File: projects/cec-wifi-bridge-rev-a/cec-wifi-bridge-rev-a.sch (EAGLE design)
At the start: 56 parts, among them J1 DX4R005HJ5R2000, J3 DEBUG, J4 10029449-001RLF, J5 PROGRAM, T1 MMBT3904, T2 MMBT3904, U1 MCP73831/2/OT, U2 TPS61200DRC, U3 ESP8266EX, U4 SPI-FLASH-SOIC8, X1 26MHz

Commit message: Add part number for ESP8266.
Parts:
- U3: PN (none) -> ESP8266EX
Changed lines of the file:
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@@
 <attribute name="BOM" value="EXCLUDE"/>
 </part>
-<part name="U3" library="espressif" deviceset="ESP8266EX" device=""/>
+<part name="U3" library="espressif" deviceset="ESP8266EX" device="">
+<attribute name="PN" value="ESP8266EX"/>
+</part>
 <part name="X1" library="crystals" deviceset="GROUNDED-CRYSTAL" device="-EPSON-TSX-3225" value="26MHz">
 <attribute name="PN" value="TSX-3225 26.0000MF09Z-AC3"/>
@@
 <attribute name="BOM" x="0" y="0" size="5.08" layer="96" display="off"/>
 </instance>
-<instance part="U3" gate="G$1" x="86.36" y="99.06"/>
+<instance part="U3" gate="G$1" x="86.36" y="99.06">
+<attribute name="PN" x="86.36" y="99.06" size="1.778" layer="96" display="off"/>
+</instance>
 <instance part="X1" gate="G$1" x="198.12" y="121.92">
 <attribute name="PN" x="198.12" y="121.92" size="1.778" layer="96" display="off"/>

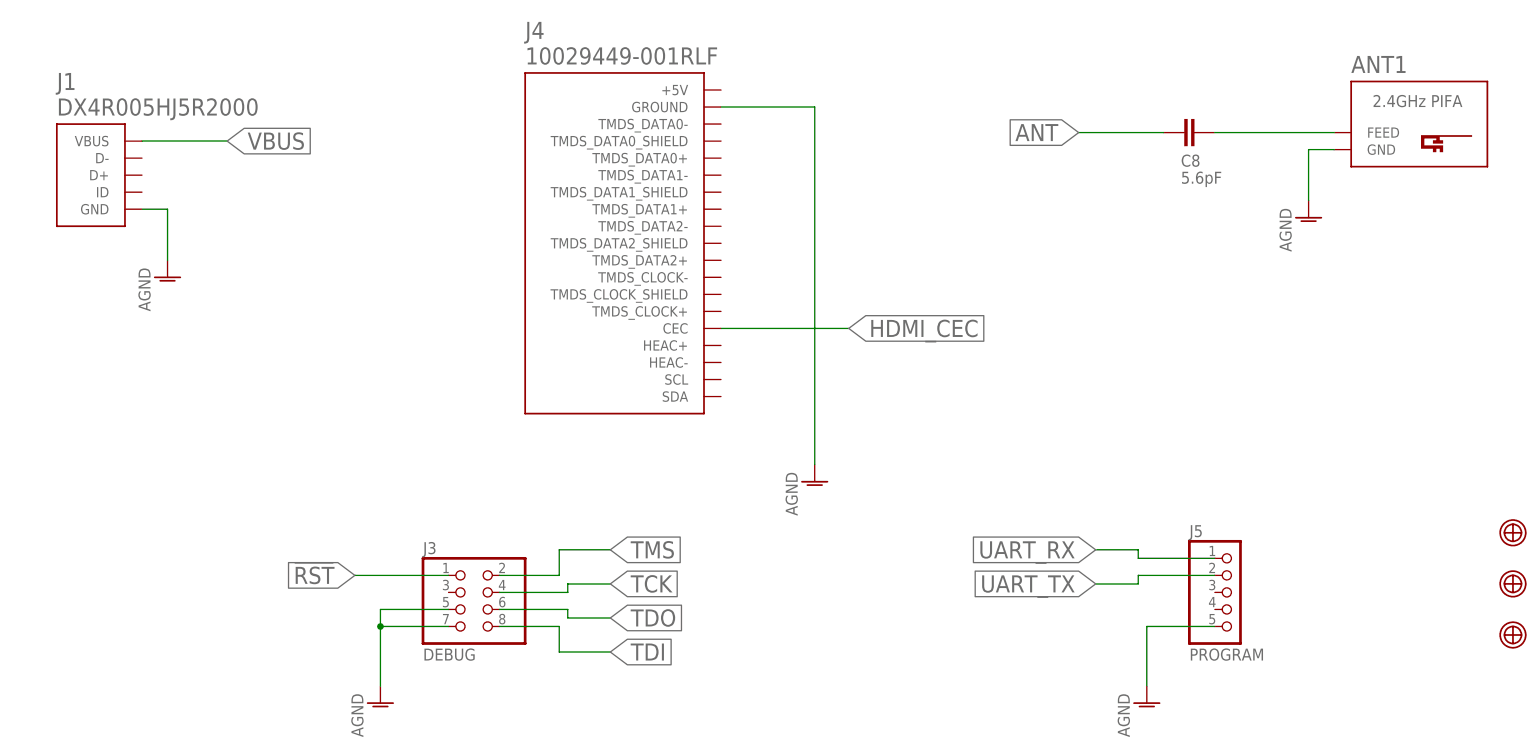
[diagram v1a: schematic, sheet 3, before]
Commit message: Add testpoints for the power rails.
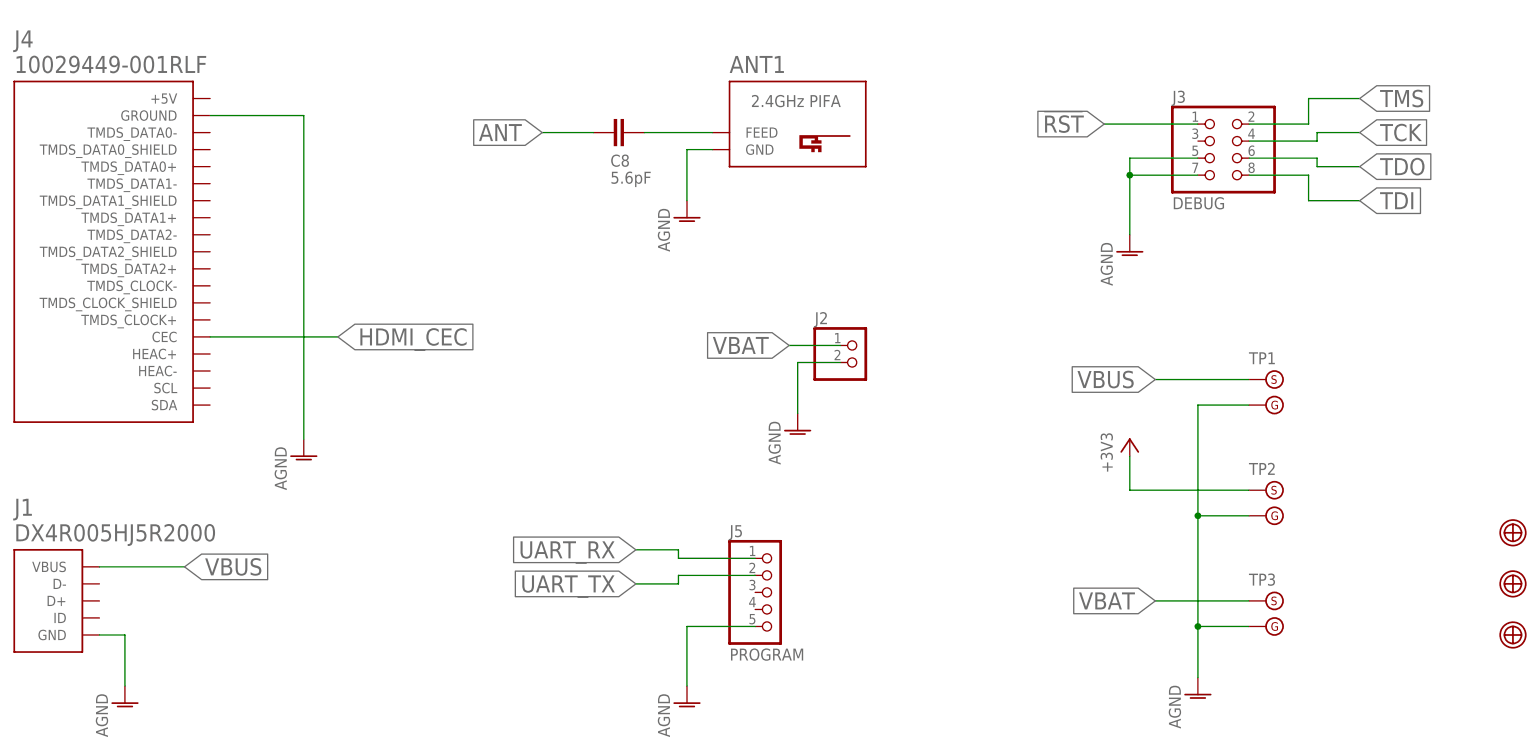
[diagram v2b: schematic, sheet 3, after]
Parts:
- added TP1, TP2, TP3: TESTPOINT-WITH-GND, test:TESTPOINT-WITH-GND
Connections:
- removed net N$1: C1.1, C3.1, J2.1, L1.2, R2.2, U1.VBAT, U2.EN, U2.PS, U2.VIN
- new net VBAT: C1.1, C3.1, J2.1, L1.2, R2.2, TP3.S, U1.VBAT, U2.EN, U2.PS, U2.VIN
- net +3V3: now also TP2.S
- net AGND: now also TP1.G, TP2.G, TP3.G
- net VBUS: now also TP1.S
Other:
- moved on the sheet: ANT1, C8, J1, J3, J4, J5

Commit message: Final layout tweaks before locking rev A.
We've given the TPS61200 its own power ground, hopefully quashing as
much noise as possible off the main ground, keeping RF performance high.

I lied, and went back to adjust the stitching.  We should have our
stitching on a 100 mil grid consistently, with a few exceptions to deal
with component placement.

Also fixed a bug where we had a decoupling cap on a configuration pin
instead of a supply pin.
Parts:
- TP1, TP2, TP3: BOM (none) -> EXCLUDE
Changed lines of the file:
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@@
 <setting verticaltext="up"/>
 </settings>
-<grid distance="0.05" unitdist="inch" unit="inch" style="lines" multiple="1" display="no" altdistance="0.01" altunitdist="inch" altunit="inch"/>
+<grid distance="0.1" unitdist="inch" unit="inch" style="lines" multiple="1" display="no" altdistance="0.01" altunitdist="inch" altunit="inch"/>
 <layers>
 <layer number="1" name="Top" color="4" fill="1" visible="no" active="no"/>
@@
 </part>
 <part name="AGND27" library="supplies" deviceset="AGND" device=""/>
-<part name="TP1" library="test" deviceset="TESTPOINT-WITH-GND" device=""/>
-<part name="TP2" library="test" deviceset="TESTPOINT-WITH-GND" device=""/>
-<part name="TP3" library="test" deviceset="TESTPOINT-WITH-GND" device=""/>
+<part name="TP1" library="test" deviceset="TESTPOINT-WITH-GND" device="">
+<attribute name="BOM" value="EXCLUDE"/>
+</part>
+<part name="TP2" library="test" deviceset="TESTPOINT-WITH-GND" device="">
+<attribute name="BOM" value="EXCLUDE"/>
+</part>
+<part name="TP3" library="test" deviceset="TESTPOINT-WITH-GND" device="">
+<attribute name="BOM" value="EXCLUDE"/>
+</part>
 <part name="AGND28" library="supplies" deviceset="AGND" device=""/>
 <part name="+3V7" library="supplies" deviceset="+3V3" device=""/>
@@
 <attribute name="BOM" x="238.76" y="25.4" size="1.778" layer="96" display="off"/>
 </instance>
-<instance part="TP1" gate="G$1" x="201.93" y="63.5"/>
-<instance part="TP2" gate="G$1" x="201.93" y="46.99"/>
-<instance part="TP3" gate="G$1" x="201.93" y="30.48"/>
+<instance part="TP1" gate="G$1" x="201.93" y="63.5">
+<attribute name="BOM" x="201.93" y="63.5" size="1.778" layer="96" display="off"/>
+</instance>
+<instance part="TP2" gate="G$1" x="201.93" y="46.99">
+<attribute name="BOM" x="201.93" y="46.99" size="1.778" layer="96" display="off"/>
+</instance>
+<instance part="TP3" gate="G$1" x="201.93" y="30.48">
+<attribute name="BOM" x="201.93" y="30.48" size="1.778" layer="96" display="off"/>
+</instance>
 <instance part="AGND28" gate="VR1" x="191.77" y="16.51"/>
 <instance part="AGND12" gate="VR1" x="132.08" y="55.88"/>
@@
 </sheet>
 </sheets>
-<errors>
-</errors>
 </schematic>
 </drawing>

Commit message: BOM tweaks to account for supply chain issues.
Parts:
- D1: PN 598-8020-107F -> APT1608SURCK
- D3: PN 598-8081-107F -> 150060GS75000
- R13: PN RC0402FR-0727KL -> ERJ-2RKF2702X
- S1, S2: PN SKQGAKE010 -> SKQGADE010
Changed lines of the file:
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@@
 <part name="AGND10" library="supplies" deviceset="AGND" device=""/>
 <part name="D1" library="dialight" deviceset="DIALIGHT-598-MICROSMD" device="-0603" value="2V, 5mA">
-<attribute name="PN" value="598-8020-107F"/>
+<attribute name="PN" value="APT1608SURCK"/>
 </part>
 <part name="R4" library="passives" deviceset="RESISTOR-HORIZONTAL" device="-0603" value="330">
@@
 <part name="+3V3" library="supplies" deviceset="+3V3" device=""/>
 <part name="S1" library="switches" deviceset="MOMENTARY" device="-ALPS-SKQG" value="RESET">
-<attribute name="PN" value="SKQGAKE010"/>
+<attribute name="PN" value="SKQGADE010"/>
 </part>
 <part name="R7" library="passives" deviceset="RESISTOR" device="-0402" value="10K">
@@
 </part>
 <part name="S2" library="switches" deviceset="MOMENTARY" device="-ALPS-SKQG" value="UPLOAD">
-<attribute name="PN" value="SKQGAKE010"/>
+<attribute name="PN" value="SKQGADE010"/>
 </part>
 <part name="AGND17" library="supplies" deviceset="AGND" device=""/>
@@
 </part>
 <part name="R13" library="passives" deviceset="RESISTOR-HORIZONTAL" device="-0402" value="27K">
-<attribute name="PN" value="RC0402FR-0727KL"/>
+<attribute name="PN" value="ERJ-2RKF2702X"/>
 </part>
 <part name="R14" library="passives" deviceset="RESISTOR-HORIZONTAL" device="-0402" value="1M">
@@
 </part>
 <part name="D3" library="dialight" deviceset="DIALIGHT-598-MICROSMD" device="-0603" value="3.2V, 5mA">
-<attribute name="PN" value="598-8081-107F"/>
+<attribute name="PN" value="150060GS75000"/>
 </part>
 <part name="AGND27" library="supplies" deviceset="AGND" device=""/>
